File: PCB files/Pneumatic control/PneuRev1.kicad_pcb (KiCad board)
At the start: 2 copper layers, 145.7 x 92.9 mm, 52 parts, among them J1 SIG_IN, J2 BATT_IN, J3 PNEU, U1 uA7824, U2 OP279, U3 OP279, U4 OP279, U5 OP279, U6 OP279, U7 OP279, U8 OP07

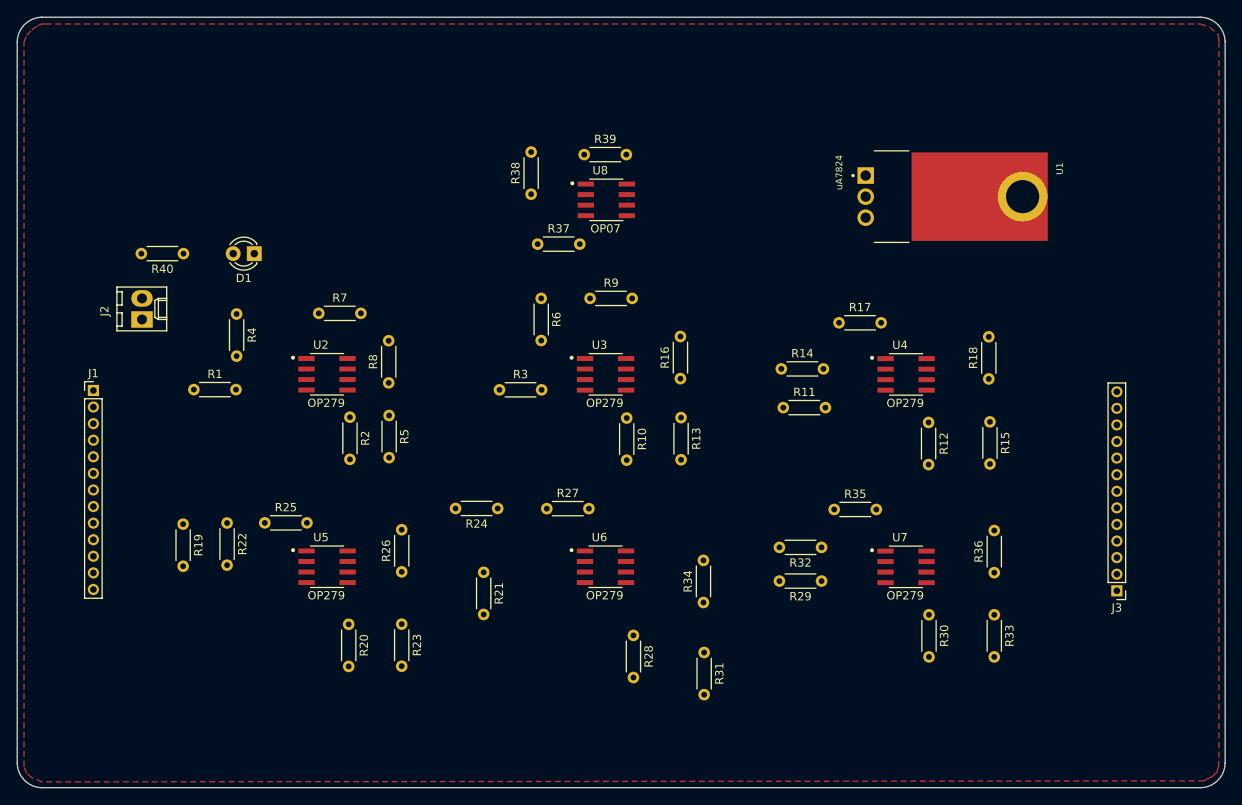
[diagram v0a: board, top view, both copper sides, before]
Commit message: 2/4/2019
-Finished board routing
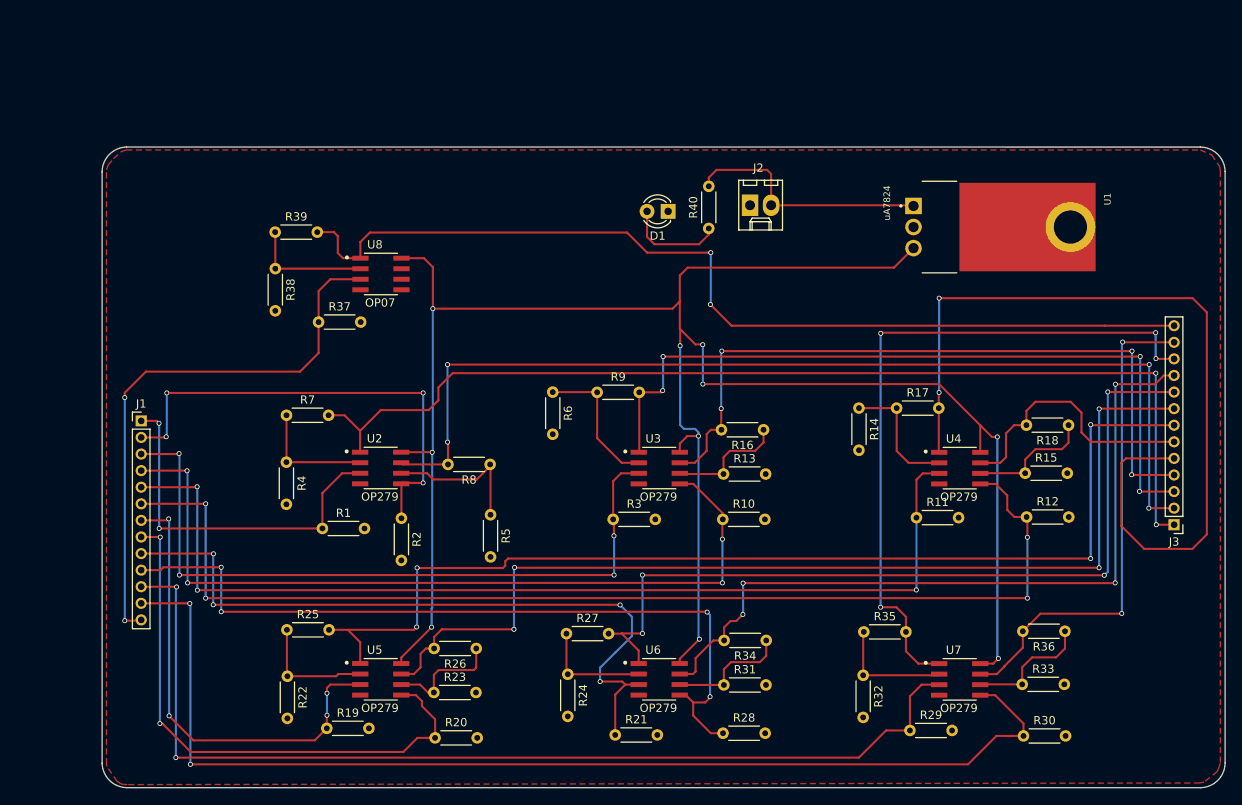
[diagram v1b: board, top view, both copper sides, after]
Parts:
- moved J2 74.6 mm to (162.6, 68.8), turned to 0 degrees
- moved R40 63.4 mm to (157.7, 71.6), turned to 90 degrees
- moved D1 50.2 mm to (152.8, 69.5)
- moved R39 38.4 mm to (105.4, 72.0)
- moved R38 32.1 mm to (105.4, 76.4), turned to 270 degrees
- moved R19 30.1 mm to (111.6, 131.9), turned to 0 degrees
- moved U8 28.6 mm to (118.1, 77.1)
- moved R37 28.0 mm to (110.6, 82.9)
- moved R21 25.2 mm to (146.4, 132.7), turned to 0 degrees
- moved R1 22.8 mm to (111.1, 107.8)
- moved R24 21.7 mm to (140.7, 125.3), turned to 270 degrees
- moved R29 20.9 mm to (181.9, 132.1), turned to 0 degrees
- moved R11 20.8 mm to (182.7, 106.5)
- moved R3 20.8 mm to (146.1, 106.7)
- moved R22 19.9 mm to (106.8, 125.6)
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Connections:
- U2 pad 1: Net-(J1-Pad1) -> /PNU1
- U2 pad 2: GND -> Net-(R4-Pad1)
- U2 pad 3: /IN2 -> Net-(J1-Pad1)
- U2 pad 4: Net-(R5-Pad1) -> GND
- U2 pad 5: /PNU2 -> /IN2
- U2 pad 6: Net-(U1-Pad3) -> Net-(R5-Pad1)
- U2 pad 7: /PNU1 -> /PNU2
- U2 pad 8: Net-(R4-Pad1) -> Net-(U1-Pad3)
- U3 pad 1: /IN3 -> /PNU3
- U3 pad 2: GND -> Net-(R6-Pad1)
- U3 pad 3: /IN4 -> /IN3
- U3 pad 4: Net-(R13-Pad1) -> GND
- U3 pad 5: /PNU4 -> /IN4
- U3 pad 6: Net-(U1-Pad3) -> Net-(R13-Pad1)
- U3 pad 7: /PNU3 -> /PNU4
- U3 pad 8: Net-(R6-Pad1) -> Net-(U1-Pad3)
- U4 pad 1: /IN5 -> /PNU5
- U4 pad 2: GND -> Net-(R14-Pad1)
- U4 pad 3: /IN6 -> /IN5
- U4 pad 4: Net-(R15-Pad1) -> GND
- U4 pad 5: /PNU6 -> /IN6
- U4 pad 6: Net-(U2-Pad6) -> Net-(R15-Pad1)
- U4 pad 7: /PNU5 -> /PNU6
- U4 pad 8: Net-(R14-Pad1) -> Net-(U1-Pad3)
- U5 pad 1: /IN7 -> /PNU7
- U5 pad 2: GND -> Net-(R22-Pad1)
- U5 pad 3: /IN8 -> /IN7
- U5 pad 4: Net-(R23-Pad1) -> GND
- U5 pad 5: /PNU8 -> /IN8
- U5 pad 6: Net-(U1-Pad3) -> Net-(R23-Pad1)
- U5 pad 7: /PNU7 -> /PNU8
- U5 pad 8: Net-(R22-Pad1) -> Net-(U1-Pad3)
- U6 pad 1: /IN9 -> /PNU9
- U6 pad 2: GND -> Net-(R24-Pad1)
- U6 pad 3: /IN10 -> /IN9
- U6 pad 4: Net-(R31-Pad1) -> GND
- U6 pad 5: /PNU10 -> /IN10
- U6 pad 6: Net-(U1-Pad3) -> Net-(R31-Pad1)
- U6 pad 7: /PNU9 -> /PNU10
- U6 pad 8: Net-(R24-Pad1) -> Net-(U1-Pad3)
- U7 pad 1: /IN11 -> /PNU11
- U7 pad 2: GND -> Net-(R32-Pad1)
- U7 pad 3: /IN12 -> /IN11
- U7 pad 4: Net-(R33-Pad1) -> GND
- U7 pad 5: /PNU12 -> /IN12
- U7 pad 6: Net-(U2-Pad6) -> Net-(R33-Pad1)
- U7 pad 7: /PNU11 -> /PNU12
- U7 pad 8: Net-(R32-Pad1) -> Net-(U1-Pad3)
- U8 pad 1: /IN13 -> /PNU13
- U8 pad 2: GND -> Net-(R38-Pad1)
- U8 pad 3: Net-(U8-Pad3) -> /IN13
- U8 pad 4: Net-(U8-Pad4) -> GND
- U8 pad 6: Net-(U1-Pad3) -> Net-(U8-Pad6)
- U8 pad 7: /PNU13 -> Net-(U8-Pad7)
- U8 pad 8: Net-(R38-Pad1) -> Net-(U1-Pad3)
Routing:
- net Net-(U1-Pad3): track 0.00 -> 249.5 mm, vias 0 -> 10
- net /IN6: track 0.00 -> 136.3 mm, vias 0 -> 4
- net /IN12: track 0.00 -> 135.3 mm, vias 0 -> 2
- net /PNU7: track 0.00 -> 130.8 mm, vias 0 -> 4
- net /PNU1: track 0.00 -> 127.3 mm, vias 0 -> 2
- net /PNU8: track 0.00 -> 123.8 mm, vias 0 -> 4
- net /IN11: track 0.00 -> 123.0 mm, vias 0 -> 2
- net /PNU2: track 0.00 -> 122.8 mm, vias 0 -> 4
- net /IN5: track 0.00 -> 122.3 mm, vias 0 -> 3
- net /PNU13: track 0.00 -> 116.6 mm, vias 0 -> 2
- net /PNU5: track 0.00 -> 104.8 mm, vias 0 -> 2
- net /PNU9: track 0.00 -> 101.6 mm, vias 0 -> 4
- net /IN4: track 0.00 -> 98.6 mm, vias 0 -> 4
- net /IN10: track 0.00 -> 94.6 mm, vias 0 -> 4
- net /PNU10: track 0.00 -> 92.6 mm, vias 0 -> 4
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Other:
- board size 145.7 x 92.9 mm -> 135.4 x 77.3 mm
